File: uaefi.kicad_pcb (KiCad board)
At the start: 4 copper layers, 135 x 125 mm, 138 parts, among them J1 211PL562L0011, J2 USB_B_Mini, J3 5569-06A2, J6 Conn_01x06, J7 Conn_01x05_Male, J9 USB_C, M1 Module-power_12and5V-0.2, M2 Module-knock-0.2, M3 Module-vr-discrete-0.5, M4 Module-vr-max9924-0.1, M5 Module-wbo-0.5, M6 Module:mega-mcu100/0.3, M7 Module-can-0.1, P1 Pad, P15 Pad, P16 Pad, P17 Pad, P18 Pad, P2 Pad, P3 Pad, P4 Pad, P7 Pad, P8 Pad, Q10 ISL9V3040D3ST, Q11 ISL9V3040D3ST, Q12 ISL9V3040D3ST, Q7 ISL9V3040D3ST, Q8 ISL9V3040D3ST, Q9 ISL9V3040D3ST, U1 TLE9201SG, U10 VNLD5160TR-E, U11 VNLD5160TR-E, U2 TLE9201SG, U3 MPX4/MPXH6400_MAP, U4 MAX31855KASA, U5 JDY-33, U6 VNLD5160TR-E, U7 VNLD5160TR-E, U8 VNLD5160TR-E, U9 VNLD5160TR-E

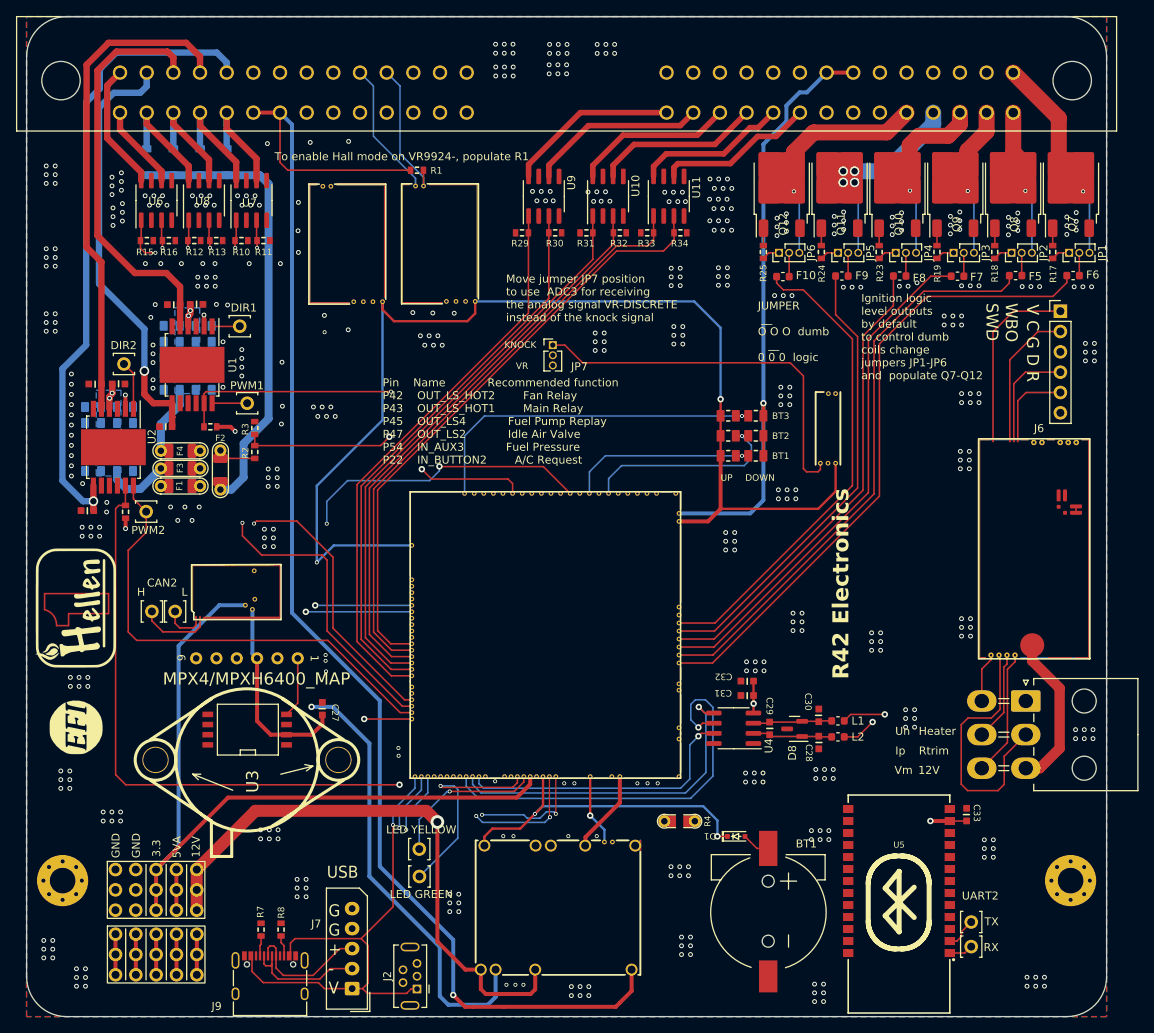
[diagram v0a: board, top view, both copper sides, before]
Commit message: Update uaefi.kicad_pcb
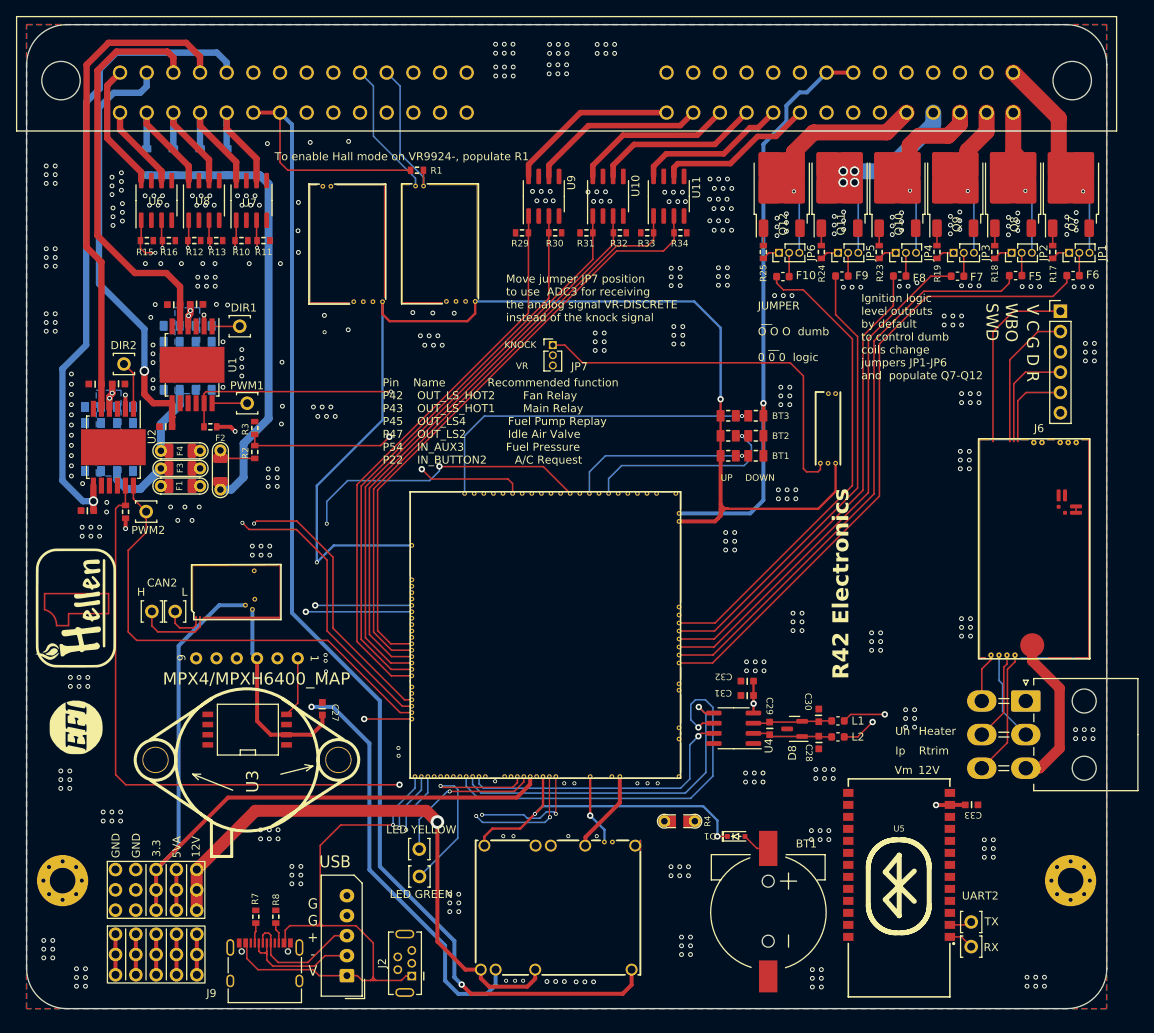
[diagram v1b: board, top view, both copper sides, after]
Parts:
- moved U5 2.02 mm to (148.5, 137.1)
- moved J2 1.74 mm to (86.8, 146.7)
- moved J7 1.74 mm to (79.5, 148.2)
- moved J9 1.74 mm to (69.3, 147.8)
- moved R7 1.74 mm to (68.1, 140.9)
- moved R8 1.74 mm to (70.6, 140.9)
- moved C33 1.37 mm to (157.6, 126.9), turned to 180 degrees
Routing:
- net /WBO_Rtrim: track 33.3 -> 11.3 mm
- net Net-(M6-UART2_TX_(PD5)): track 82.7 -> 69.8 mm
- net /VBUS: track 64.5 -> 71.8 mm
- net Net-(M6-UART2_RX_(PD6)): track 70.5 -> 76.5 mm
- net +3.3V: track 137.6 -> 143.1 mm
- net +3.3VA: track 168.9 -> 173.5 mm
- net /IN_VIGN: track 95.2 -> 91.7 mm
- net +5VA: track 249.8 -> 253.0 mm
- net +5VP: track 172.0 -> 168.8 mm
- net +12V_RAW: track 269.9 -> 267.6 mm
- net /USB-: track 50.8 -> 49.6 mm
- net /DC1_DIR: track 65.9 -> 64.9 mm
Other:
- board size 135 x 125 mm -> 135 x 123 mm
